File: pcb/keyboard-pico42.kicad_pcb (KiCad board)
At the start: 2 copper layers, 227 x 75 mm, 90 parts, among them U1 Pico

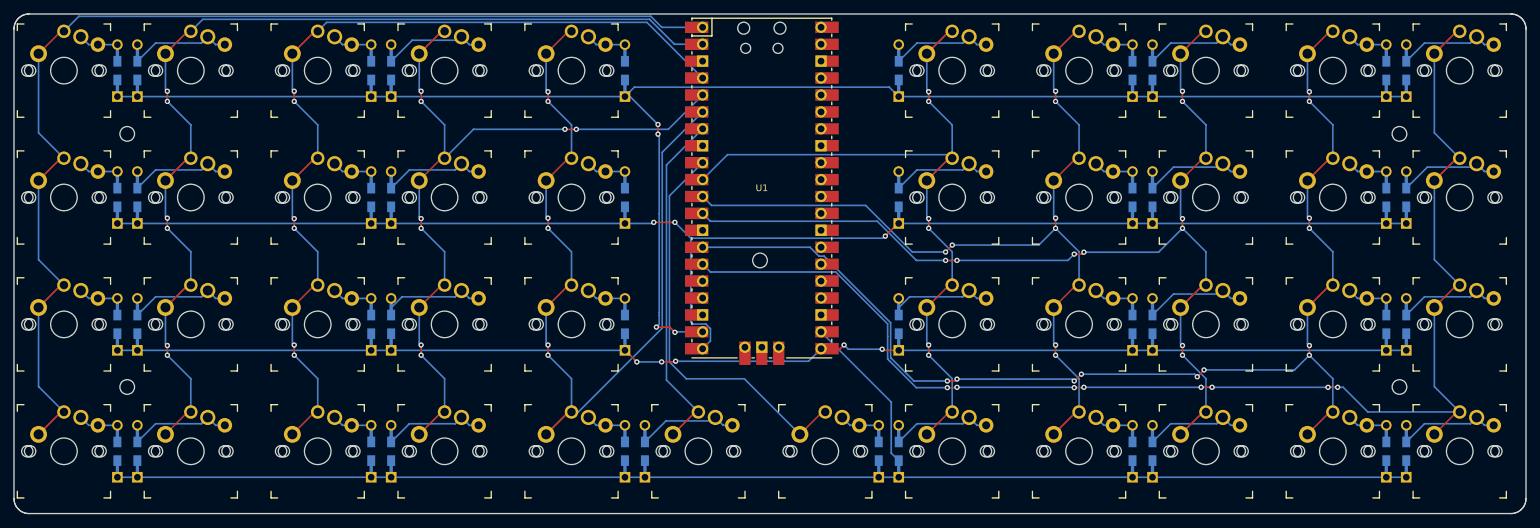
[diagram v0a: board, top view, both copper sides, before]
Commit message: pcb: pico42 rev2023.2
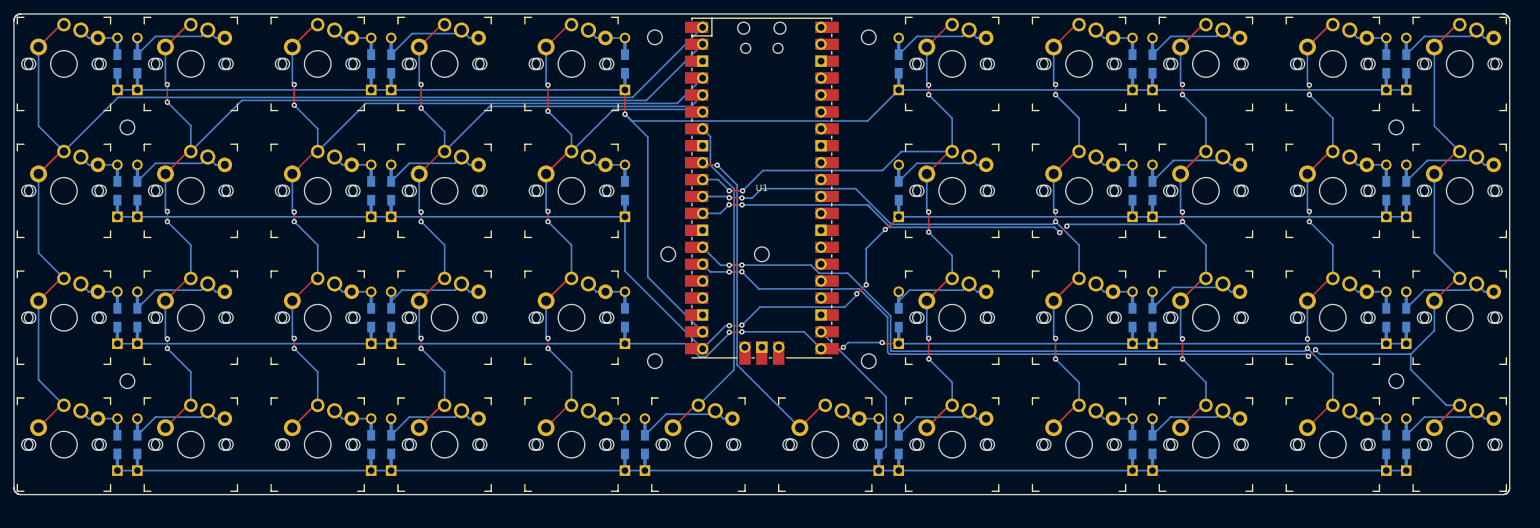
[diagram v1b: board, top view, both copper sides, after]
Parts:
- added H10: MountingHole, MountingHole:MountingHole_2.2mm_M2_DIN965, F.Cu at (178.3, 53.5)
- added H6: MountingHole, MountingHole:MountingHole_2.2mm_M2_DIN965, F.Cu at (148.2, 86.1)
- added H7: MountingHole, MountingHole:MountingHole_2.2mm_M2_DIN965, F.Cu at (146.2, 53.5)
- added H8: MountingHole, MountingHole:MountingHole_2.2mm_M2_DIN965, F.Cu at (146.2, 102.1)
- added H9: MountingHole, MountingHole:MountingHole_2.2mm_M2_DIN965, F.Cu at (178.3, 102.1)
- moved H2 194.6 mm to (67.0, 105.1)
- moved H3 190.5 mm to (257.5, 105.1)
- moved H4 39.0 mm to (257.5, 67.0)
- moved D_1_1 1.00 mm to (65.5, 57.5)
- moved D_1_10 1.00 mm to (220.9, 57.5)
- moved D_1_11 1.00 mm to (256.0, 57.5)
- moved D_1_12 1.00 mm to (259.0, 57.5)
- moved D_1_2 1.00 mm to (68.5, 57.5)
- moved D_1_3 1.00 mm to (103.6, 57.5)
- moved D_1_4 1.00 mm to (106.6, 57.5)
- moved D_1_5 1.00 mm to (141.7, 57.5)
- moved D_1_8 1.00 mm to (182.8, 57.5)
- moved D_1_9 1.00 mm to (217.9, 57.5)
- moved D_2_1 1.00 mm to (65.5, 76.5)
- moved D_2_10 1.00 mm to (220.9, 76.5)
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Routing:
- net /COL5: track 126.4 -> 93.3 mm
- net /COL7: track 61.3 -> 51.1 mm, vias 0 -> 1
- net /COL12: track 198.6 -> 190.7 mm, vias 8 -> 4
- net /COL11: track 177.3 -> 171.4 mm, vias 12 -> 8
- net /COL1: track 170.1 -> 174.4 mm
- net /COL9: track 130.5 -> 126.9 mm
- net /COL10: track 149.6 -> 146.2 mm
- net /ROW2: track 214.9 -> 218.0 mm, vias 3 -> 5
- net /COL2: track 151.7 -> 154.3 mm
- net /ROW1: track 239.3 -> 237.0 mm, vias 4 -> 1
- net /COL4: track 115.3 -> 113.1 mm, vias 8 -> 6
- net /ROW3: track 195.6 -> 197.5 mm, vias 5 -> 4
- net /COL6: track 51.9 -> 50.4 mm
- net /ROW4: track 217.7 -> 216.3 mm
- net /COL3: track 134.4 -> 133.2 mm
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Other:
- board size 227 x 75 mm -> 224.6 x 72.2 mm
